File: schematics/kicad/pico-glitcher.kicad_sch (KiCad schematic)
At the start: 72 parts, among them Q1 IRLML2502, Q2 IRF7807PBF, Q3 TPS 79318, Q4 TPS2041, U1 NH245, U2 NH245, X1 BU-SMA-V, X2 BU-SMA, X3 M08X2

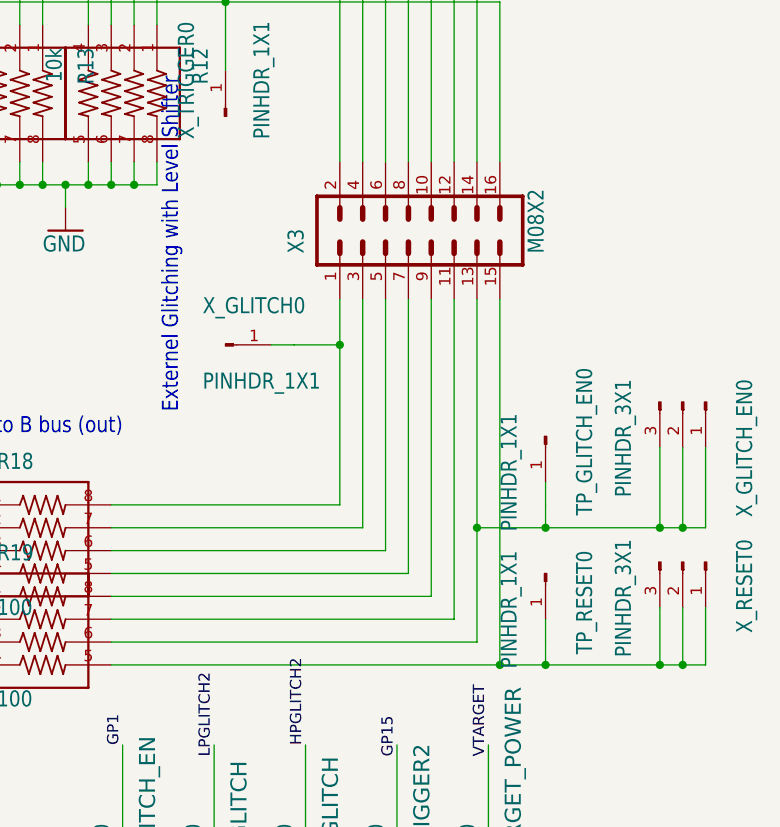
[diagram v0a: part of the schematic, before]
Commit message: replaced 2x08 pinheader's symbol and footprint with kicad library's ones
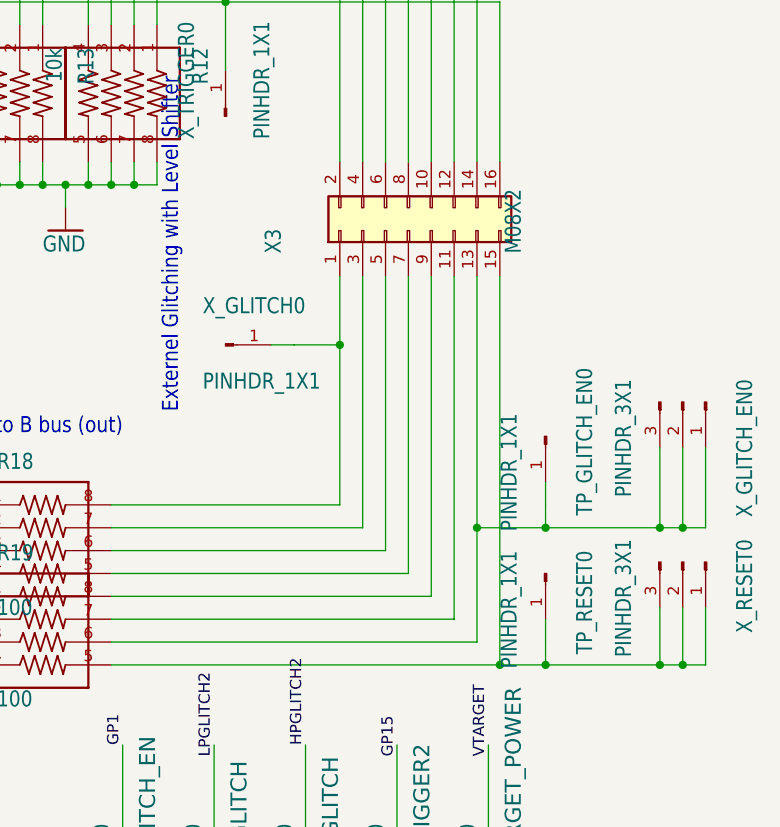
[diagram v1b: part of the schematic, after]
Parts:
- X3: footprint pico-glitcher:2X8 -> Connector_PinHeader_2.54mm:PinHeader_2x08_P2.54mm_Vertical; symbol pico-glitcher:M08X2 -> Connector_Generic:Conn_02x08_Odd_Even
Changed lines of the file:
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@@
 	(wire
 		(pts
-			(xy 266.7 175.26) (xy 266.7 144.78)
+			(xy 266.7 175.26) (xy 266.7 142.24)
 		)
 		(stroke
@@
 	(wire
 		(pts
-			(xy 276.86 185.42) (xy 276.86 144.78)
+			(xy 276.86 185.42) (xy 276.86 142.24)
 		)
 		(stroke
@@
 	(wire
 		(pts
-			(xy 264.16 172.72) (xy 264.16 144.78)
+			(xy 264.16 172.72) (xy 264.16 142.24)
 		)
 		(stroke
@@
 	(wire
 		(pts
-			(xy 259.08 144.78) (xy 259.08 149.86)
+			(xy 259.08 142.24) (xy 259.08 149.86)
 		)
 		(stroke
@@
 	(wire
 		(pts
-			(xy 261.62 170.18) (xy 261.62 144.78)
+			(xy 261.62 170.18) (xy 261.62 142.24)
 		)
 		(stroke
@@
 	(wire
 		(pts
-			(xy 271.78 180.34) (xy 271.78 144.78)
+			(xy 271.78 180.34) (xy 271.78 142.24)
 		)
 		(stroke
@@
 	(wire
 		(pts
-			(xy 269.24 177.8) (xy 269.24 144.78)
+			(xy 269.24 177.8) (xy 269.24 142.24)
 		)
 		(stroke
@@
 	(wire
 		(pts
-			(xy 274.32 170.18) (xy 274.32 144.78)
+			(xy 274.32 170.18) (xy 274.32 142.24)
 		)
 		(stroke
@@
 	)
 	(symbol
-		(lib_id "pico-glitcher:M08X2")
-		(at 269.24 137.16 90)
+		(lib_id "Connector_Generic:Conn_02x08_Odd_Even")
+		(at 266.7 137.16 90)
 		(unit 1)
 		(exclude_from_sim no)
@@
 		(dnp no)
 		(property "Reference" "X3"
-			(at 255.27 139.7 0)
+			(at 252.73 139.7 0)
 			(effects
 				(font
@@
 		)
 		(property "Value" "M08X2"
-			(at 281.94 139.7 0)
+			(at 279.4 139.7 0)
 			(effects
 				(font
@@
 			)
 		)
-		(property "Footprint" "pico-glitcher:2X8"
-			(at 269.24 137.16 0)
+		(property "Footprint" "Connector_PinHeader_2.54mm:PinHeader_2x08_P2.54mm_Vertical"
+			(at 266.7 137.16 0)
 			(effects
 				(font
@@
 			)
 		)
-		(property "Datasheet" ""
-			(at 269.24 137.16 0)
+		(property "Datasheet" "~"
+			(at 266.7 137.16 0)
 			(effects
 				(font
@@
 			)
 		)
-		(property "Description" ""
-			(at 269.24 137.16 0)
+		(property "Description" "Generic connector, double row, 02x08, odd/even pin numbering scheme (row 1 odd numbers, row 2 even numbers), script generated (kicad-library-utils/schlib/autogen/connector/)"
+			(at 266.7 137.16 0)
 			(effects
 				(font
